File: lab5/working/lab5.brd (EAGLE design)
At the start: 133.9 x 134 mm, 52 parts, among them J1 ISP, Q1 FET, Q2 FET, Q3 FET, Q4 FET, U1 ATMEGA128RFA1, Y1 16MHz

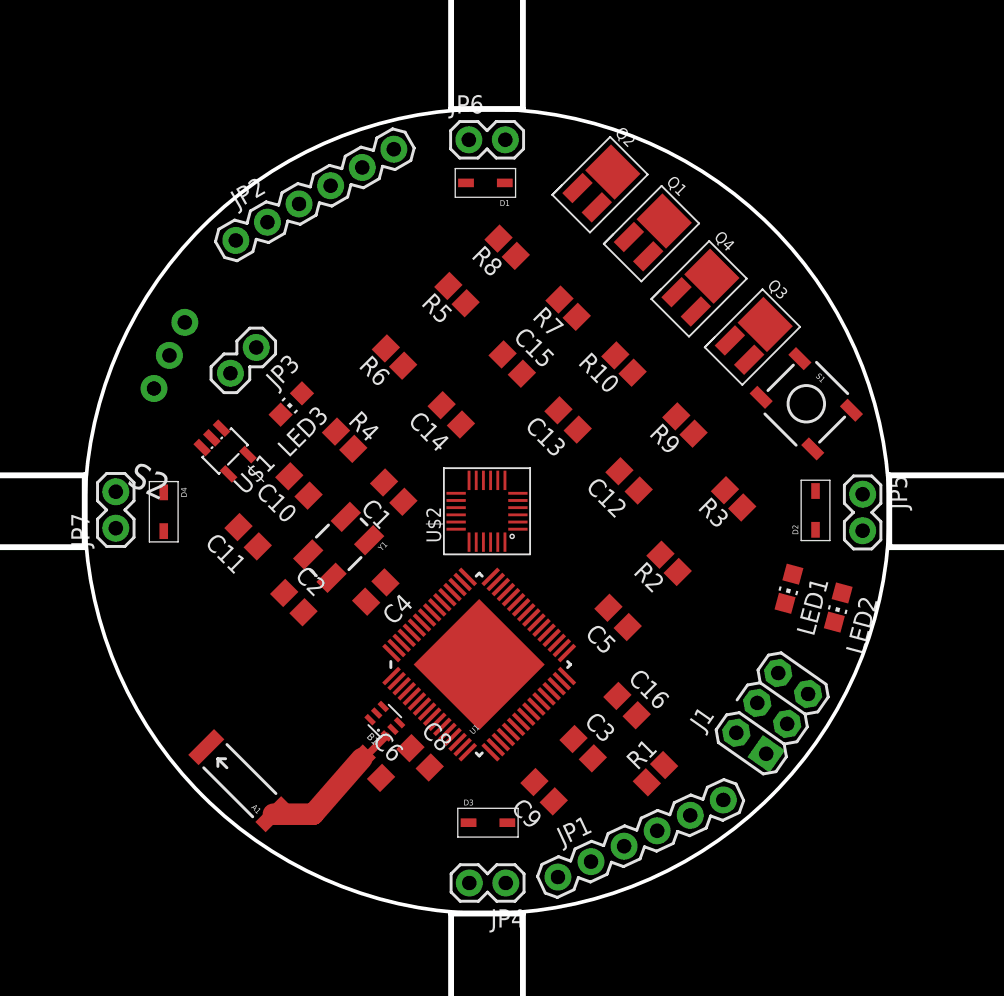
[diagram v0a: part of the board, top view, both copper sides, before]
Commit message: fixed radio
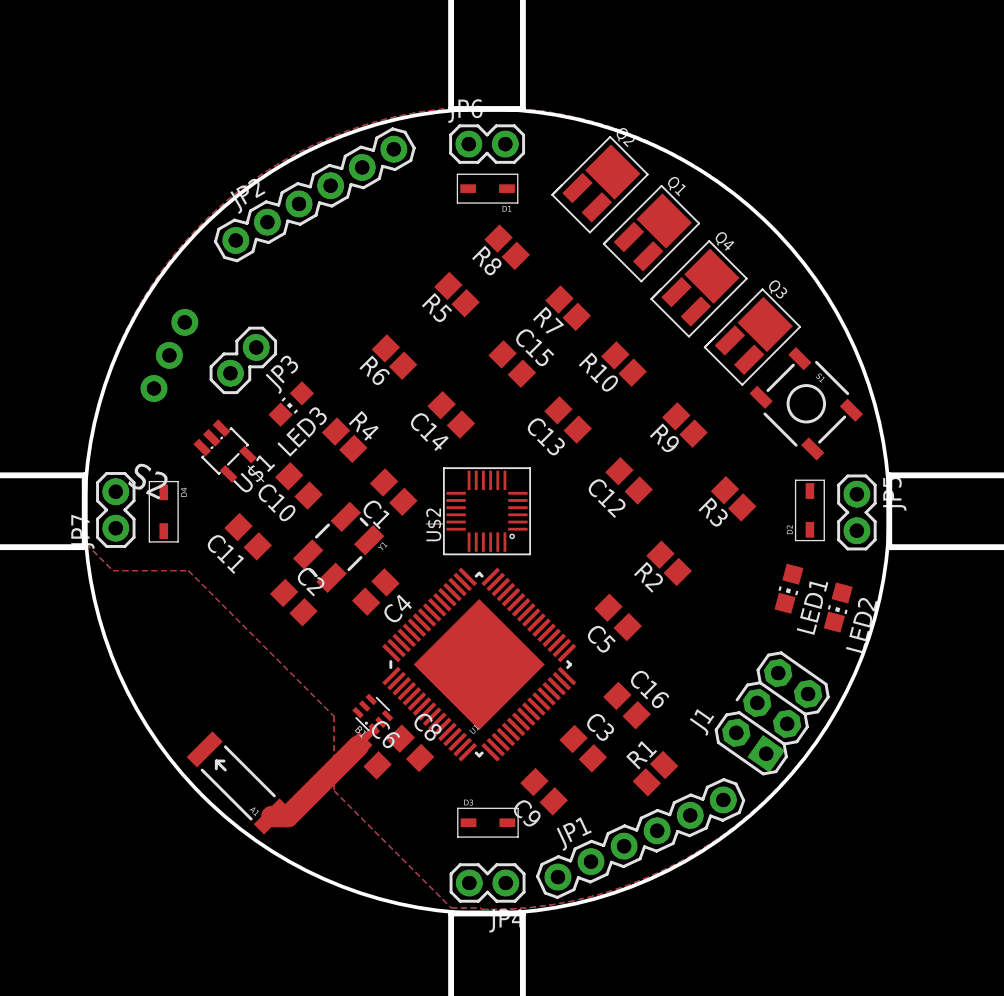
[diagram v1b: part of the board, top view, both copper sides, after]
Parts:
- moved B1 0.97 mm to (-7.95, -14.1)
- moved C8 0.94 mm to (-5.33, -16.5)
- moved C6 0.90 mm to (-8.29, -17.0)
- moved D1 0.43 mm to (0.04, 22.5)
- moved JP5 0.40 mm to (25.7, 1.19)
- moved D2 0.39 mm to (22.5, 0.06)
- moved JP6 0.30 mm to (-1.26, 25.6)
- moved A1 0.19 mm to (-17.3, -18.9)
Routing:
- net N$4: track 10.3 -> 9.71 mm
- added copper zone on layer 1, net GND
- added copper zone on layer 16, net GND
